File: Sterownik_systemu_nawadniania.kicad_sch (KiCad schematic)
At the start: 0 parts

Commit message: MCU + ESP
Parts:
- added C? (x2): 4.7uF, symbol Device:C
- added C?: 10nF, symbol Device:C
- added C? (x2): 100nF, symbol Device:C
- added C? (x2): 14pF, symbol Device:C
- added C? (x3): 1uF, symbol Device:C
- added IC?: STM32F030C6T6, QFP50P900X900X160-48N, symbol STM32F030C6T6:STM32F030C6T6
- added R?: 1.5k, symbol Device:R
- added R? (x5): 10k, symbol Device:R
- added U?: ESP-12E, RF_Module:ESP-12E, symbol RF_Module:ESP-12E
- added Y?: Crystal, symbol Device:Crystal
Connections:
- new net: C?.2, IC?.5 (PF0-OSC_IN), Y?.1
- new net: C?.2, R?.1, Y?.2
- new net: IC?.6 (PF1-OSC_OUT), R?.2
- new net: R?.1, U?.16 (GPIO15)
- new net: R?.1, U?.17 (GPIO2)
- new net: R?.1, U?.18 (GPIO0)
- new net: R?.2, U?.3 (EN)
- new net Btn_1: IC?.15 (PA5)
- new net Btn_2: IC?.16 (PA6)
- new net Btn_3: IC?.17 (PA7)
- new net Btn_4: IC?.18 (PB0)
- new net Btn_5: IC?.19 (PB1)
- new net Btn_6: IC?.20 (PB2)
- new net DISP_DB0: IC?.27 (PB14)
- new net DISP_DB1: IC?.28 (PB15)
- new net DISP_DB2: IC?.29 (PA8)
- new net DISP_DB3: IC?.30 (PA9)
- new net DISP_DB4: IC?.31 (PA10)
- new net DISP_DB5: IC?.32 (PA11)
- new net DISP_DB6: IC?.33 (PA12)
- new net DISP_DB7: IC?.35 (PF6)
- new net DISP_E: IC?.26 (PB13)
- new net DISP_RS: IC?.22 (PB11)
- new net DISP_RW: IC?.25 (PB12)
- new net ESP_NRST: C?.1, IC?.14 (PA4), R?.2, U?.1 (~{RST})
- new net GND: C?.1, C?.1, C?.2, C?.2, C?.2, C?.2, C?.2, C?.2, C?.2, C?.2, IC?.23 (VSS_1), IC?.44 (BOOT0), IC?.47 (VSS_2), IC?.8 (VSSA), R?.2, U?.15 (GND)
- new net NRST: C?.1, IC?.7 (NRST)
- new net Rain_Sensor: IC?.21 (PB10)
- new net SWCLK: IC?.37 (PA14)
- new net SWDIO: IC?.34 (PA13)
- new net USART1_Rx: IC?.13 (PA3), U?.22 (GPIO1/TXD)
- new net USART1_Tx: IC?.12 (PA2), U?.21 (GPIO3/RXD)
- new net VDD: C?.1, C?.1, C?.1, C?.1, IC?.1 (VDD_1), IC?.24 (VDD_2), IC?.48 (VDD_3), R?.1, R?.1, R?.2, R?.2, U?.8 (VCC)
- new net VDDA: C?.1, C?.1, IC?.9 (VDDA)
- new net Valve_1: IC?.39 (PB3)
- new net Valve_2: IC?.40 (PB4)
- new net Valve_3: IC?.41 (PB5)
- new net Valve_4: IC?.42 (PB6)
- no-connect marks 0 -> 23

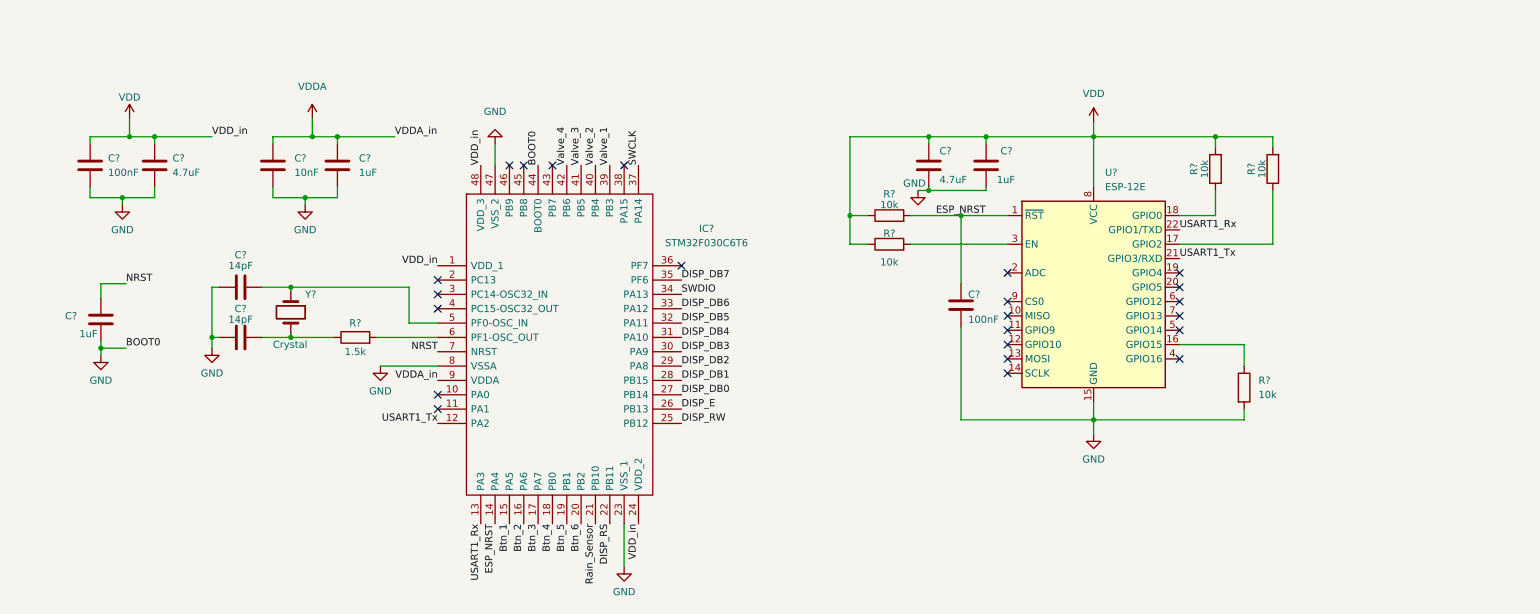
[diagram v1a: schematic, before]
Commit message: Connectors
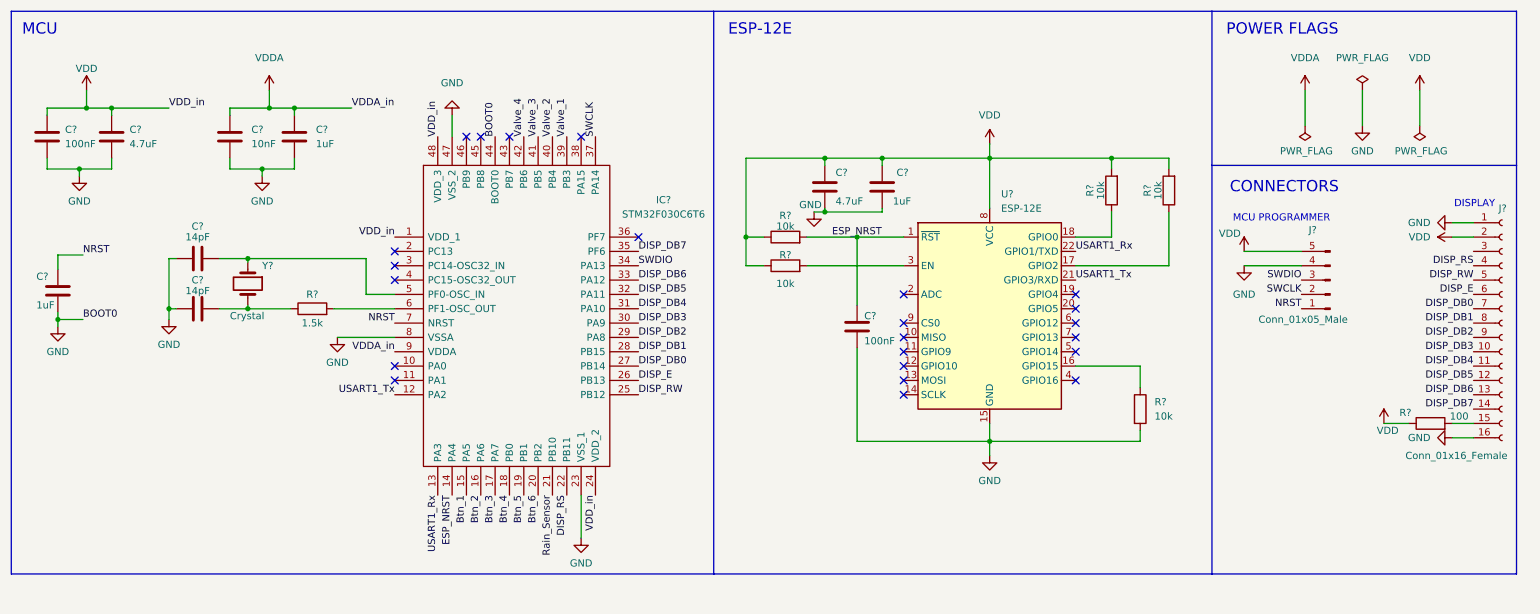
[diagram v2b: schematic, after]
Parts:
- added J?: Conn_01x05_Male, symbol Connector:Conn_01x05_Male
- added J?: Conn_01x16_Female, symbol Connector:Conn_01x16_Female
- added R?: 100, symbol Device:R
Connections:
- net DISP_DB0: now also J?.7 (Pin_7)
- net DISP_DB1: now also J?.8 (Pin_8)
- net DISP_DB2: now also J?.9 (Pin_9)
- net DISP_DB3: now also J?.10 (Pin_10)
- net DISP_DB4: now also J?.11 (Pin_11)
- net DISP_DB5: now also J?.12 (Pin_12)
- net DISP_DB6: now also J?.13 (Pin_13)
- net DISP_DB7: now also J?.14 (Pin_14)
- net DISP_E: now also J?.6 (Pin_6)
- net DISP_RS: now also J?.4 (Pin_4)
- net DISP_RW: now also J?.5 (Pin_5)
- net GND: now also J?.1 (Pin_1), J?.16 (Pin_16), J?.4 (Pin_4)
- net NRST: now also J?.1 (Pin_1)
- net SWCLK: now also J?.2 (Pin_2)
- net SWDIO: now also J?.3 (Pin_3)
- net VDD: now also J?.2 (Pin_2), J?.5 (Pin_5), R?.1
- new net: J?.15 (Pin_15), R?.2
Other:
- note added: "CONNECTORS"
- note added: "DISPLAY"
- note added: "ESP-12E"
- note added: "MCU"
- note added: "MCU PROGRAMMER"
- note added: "POWER FLAGS"
- moved on the sheet: C?, IC?, R?, U?, Y?
